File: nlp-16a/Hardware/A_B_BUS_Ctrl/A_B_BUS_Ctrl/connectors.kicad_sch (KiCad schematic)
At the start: 2 parts

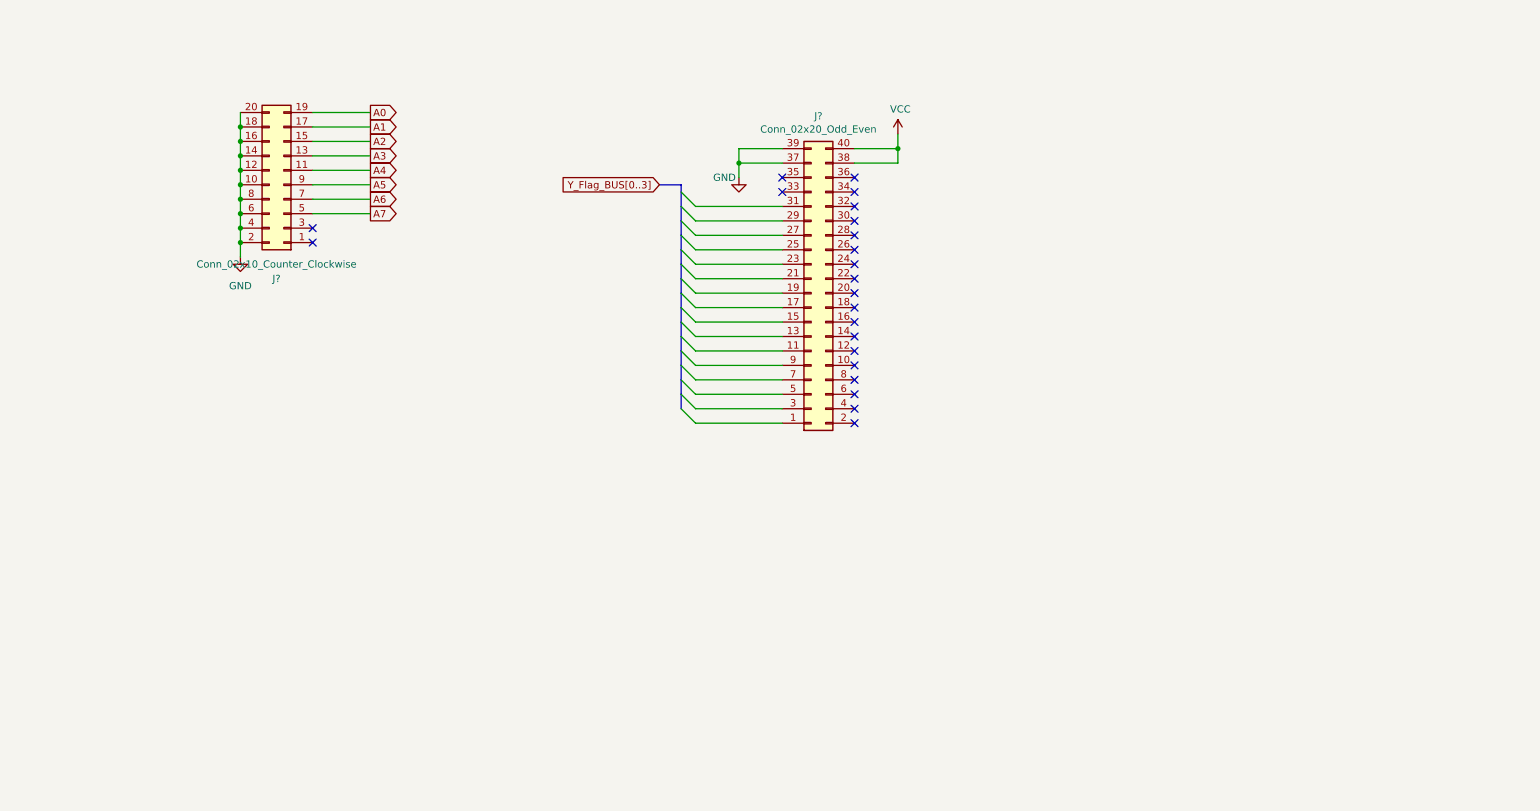
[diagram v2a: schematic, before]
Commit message: 配線作業開始
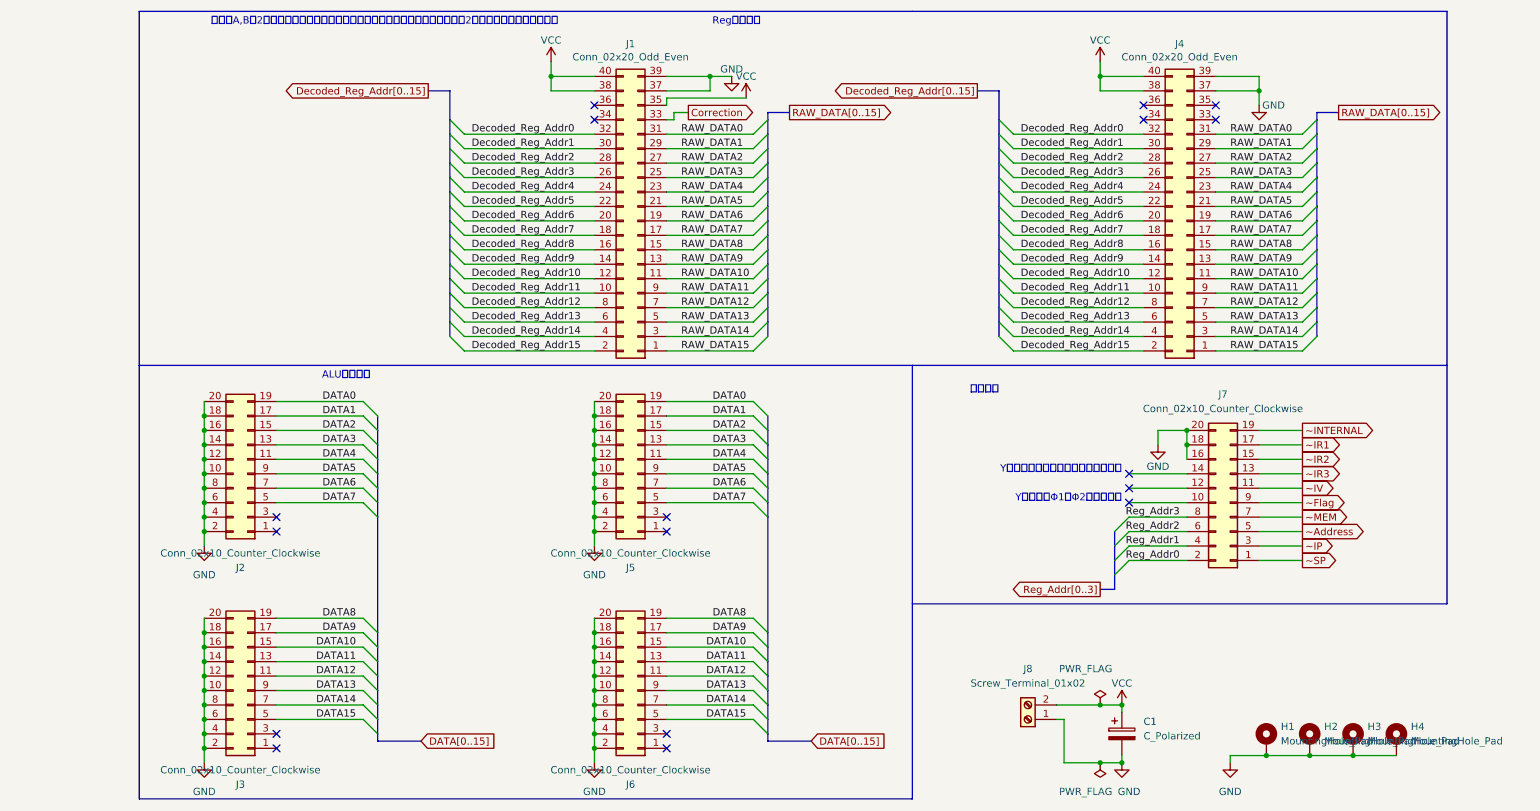
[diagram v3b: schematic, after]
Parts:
- added C1: C_Polarized, Capacitor_THT:CP_Radial_D5.0mm_P2.50mm, symbol Device:C_Polarized
- added H1, H2, H3, H4: MountingHole_Pad, MountingHole:MountingHole_3mm_Pad, symbol Mechanical:MountingHole_Pad
- added J3, J5, J6, J7: Conn_02x10_Counter_Clockwise, Connector_PinHeader_2.54mm:PinHeader_2x10_P2.54mm_Horizontal, symbol Connector_Generic:Conn_02x10_Odd_Even
- added J4: Conn_02x20_Odd_Even, Connector_PinHeader_2.54mm:PinHeader_2x20_P2.54mm_Horizontal, symbol Connector_Generic:Conn_02x20_Odd_Even
- added J8: Screw_Terminal_01x02, TerminalBlock:TerminalBlock_bornier-2_P5.08mm, symbol Connector:Screw_Terminal_01x02
- gave numbers to parts that had none: 2
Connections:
- net GND: now also C1.2, H1.1, H2.1, H3.1, H4.1, J3.10 (Pin_10), J3.12 (Pin_12), J3.14 (Pin_14), J3.16 (Pin_16), J3.18 (Pin_18), J3.2 (Pin_2), J3.20 (Pin_20), J3.4 (Pin_4), J3.6 (Pin_6), J3.8 (Pin_8), J4.37 (Pin_37), J4.39 (Pin_39), J5.10 (Pin_10), J5.12 (Pin_12), J5.14 (Pin_14), J5.16 (Pin_16), J5.18 (Pin_18), J5.2 (Pin_2), J5.20 (Pin_20), J5.4 (Pin_4), J5.6 (Pin_6), J5.8 (Pin_8), J6.10 (Pin_10), J6.12 (Pin_12), J6.14 (Pin_14), J6.16 (Pin_16), J6.18 (Pin_18), J6.2 (Pin_2), J6.20 (Pin_20), J6.4 (Pin_4), J6.6 (Pin_6), J6.8 (Pin_8), J7.16 (Pin_16), J7.18 (Pin_18), J7.20 (Pin_20), J8.1 (Pin_1)
- net VCC: now also J1.35 (Pin_35), C1.1, J4.38 (Pin_38), J4.40 (Pin_40), J8.2 (Pin_2)
- net RAW_DATA15: now reaches J1.1 (Pin_1)
- net RAW_DATA15: now also J4.1 (Pin_1)
- net Decoded_Reg_Addr11: now reaches J1.10 (Pin_10)
- net Decoded_Reg_Addr11: now also J4.10 (Pin_10)
- net RAW_DATA10: now reaches J1.11 (Pin_11)
- net RAW_DATA10: now also J4.11 (Pin_11)
- net Decoded_Reg_Addr10: now reaches J1.12 (Pin_12)
- net Decoded_Reg_Addr10: now also J4.12 (Pin_12)
- net RAW_DATA9: now reaches J1.13 (Pin_13)
- net RAW_DATA9: now also J4.13 (Pin_13)
- net Decoded_Reg_Addr9: now reaches J1.14 (Pin_14)
- net Decoded_Reg_Addr9: now also J4.14 (Pin_14)
- net RAW_DATA8: now reaches J1.15 (Pin_15)
- net RAW_DATA8: now also J4.15 (Pin_15)
- net Decoded_Reg_Addr8: now reaches J1.16 (Pin_16)
- net Decoded_Reg_Addr8: now also J4.16 (Pin_16)
- net RAW_DATA7: now reaches J1.17 (Pin_17)
- net RAW_DATA7: now also J4.17 (Pin_17)
- net Decoded_Reg_Addr7: now reaches J1.18 (Pin_18)
- net Decoded_Reg_Addr7: now also J4.18 (Pin_18)
- net RAW_DATA6: now reaches J1.19 (Pin_19)
- net RAW_DATA6: now also J4.19 (Pin_19)
- net Decoded_Reg_Addr15: now reaches J1.2 (Pin_2)
- net Decoded_Reg_Addr15: now also J4.2 (Pin_2)
- net Decoded_Reg_Addr6: now reaches J1.20 (Pin_20)
- net Decoded_Reg_Addr6: now also J4.20 (Pin_20)
- net RAW_DATA5: now reaches J1.21 (Pin_21)
- net RAW_DATA5: now also J4.21 (Pin_21)
- net Decoded_Reg_Addr5: now reaches J1.22 (Pin_22)
- net Decoded_Reg_Addr5: now also J4.22 (Pin_22)
- net RAW_DATA4: now reaches J1.23 (Pin_23)
- net RAW_DATA4: now also J4.23 (Pin_23)
- net Decoded_Reg_Addr4: now reaches J1.24 (Pin_24)
- net Decoded_Reg_Addr4: now also J4.24 (Pin_24)
- net RAW_DATA3: now reaches J1.25 (Pin_25)
- net RAW_DATA3: now also J4.25 (Pin_25)
- net Decoded_Reg_Addr3: now reaches J1.26 (Pin_26)
- net Decoded_Reg_Addr3: now also J4.26 (Pin_26)
- net RAW_DATA2: now reaches J1.27 (Pin_27)
- net RAW_DATA2: now also J4.27 (Pin_27)
- net Decoded_Reg_Addr2: now reaches J1.28 (Pin_28)
- net Decoded_Reg_Addr2: now also J4.28 (Pin_28)
- net RAW_DATA1: now reaches J1.29 (Pin_29)
- net RAW_DATA1: now also J4.29 (Pin_29)
- net RAW_DATA14: now reaches J1.3 (Pin_3)
- net RAW_DATA14: now also J4.3 (Pin_3)
- net Decoded_Reg_Addr1: now reaches J1.30 (Pin_30)
- net Decoded_Reg_Addr1: now also J4.30 (Pin_30)
- net RAW_DATA0: now reaches J1.31 (Pin_31)
- net RAW_DATA0: now also J4.31 (Pin_31)
- net Decoded_Reg_Addr0: now reaches J1.32 (Pin_32)
- net Decoded_Reg_Addr0: now also J4.32 (Pin_32)
- net Correction: now reaches J1.33 (Pin_33)
- net Decoded_Reg_Addr14: now reaches J1.4 (Pin_4)
- net Decoded_Reg_Addr14: now also J4.4 (Pin_4)
- net RAW_DATA13: now reaches J1.5 (Pin_5)
- net RAW_DATA13: now also J4.5 (Pin_5)
- net Decoded_Reg_Addr13: now reaches J1.6 (Pin_6)
- net Decoded_Reg_Addr13: now also J4.6 (Pin_6)
- net RAW_DATA12: now reaches J1.7 (Pin_7)
- net RAW_DATA12: now also J4.7 (Pin_7)
- net Decoded_Reg_Addr12: now reaches J1.8 (Pin_8)
- net Decoded_Reg_Addr12: now also J4.8 (Pin_8)
- net RAW_DATA11: now reaches J1.9 (Pin_9)
- net RAW_DATA11: now also J4.9 (Pin_9)
- net A0 renamed DATA0
- net DATA0: now also J5.19 (Pin_19)
- net A1 renamed DATA1
- net DATA1: now also J5.17 (Pin_17)
- net A2 renamed DATA2
- net DATA2: now also J5.15 (Pin_15)
- net A3 renamed DATA3
- net DATA3: now also J5.13 (Pin_13)
- net A4 renamed DATA4
- net DATA4: now also J5.11 (Pin_11)
- net A5 renamed DATA5
- net DATA5: now also J5.9 (Pin_9)
- net A6 renamed DATA6
- net DATA6: now also J5.7 (Pin_7)
- net A7 renamed DATA7
- net DATA7: now also J5.5 (Pin_5)
- new net DATA10: J3.15 (Pin_15), J6.15 (Pin_15)
- new net DATA11: J3.13 (Pin_13), J6.13 (Pin_13)
- new net DATA12: J3.11 (Pin_11), J6.11 (Pin_11)
- new net DATA13: J3.9 (Pin_9), J6.9 (Pin_9)
- new net DATA14: J3.7 (Pin_7), J6.7 (Pin_7)
- new net DATA15: J3.5 (Pin_5), J6.5 (Pin_5)
- new net DATA8: J3.19 (Pin_19), J6.19 (Pin_19)
- new net DATA9: J3.17 (Pin_17), J6.17 (Pin_17)
- new net Reg_Addr0: J7.2 (Pin_2)
- new net Reg_Addr1: J7.4 (Pin_4)
- new net Reg_Addr2: J7.6 (Pin_6)
- new net Reg_Addr3: J7.8 (Pin_8)
- new net ~Address: J7.5 (Pin_5)
- new net ~Flag: J7.9 (Pin_9)
- new net ~INTERNAL: J7.19 (Pin_19)
- new net ~IP: J7.3 (Pin_3)
- new net ~IR1: J7.17 (Pin_17)
- new net ~IR2: J7.15 (Pin_15)
- new net ~IR3: J7.13 (Pin_13)
- new net ~IV: J7.11 (Pin_11)
- new net ~MEM: J7.7 (Pin_7)
- new net ~SP: J7.1 (Pin_1)
- no-connect marks 22 -> 17
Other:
- note added: "ALUバス出力"
- note added: "Regバス入力"
- note added: "YバスではΦ1，Φ2で使用する"
- note added: "Yバスでは全レジスタ指定で使用する"
- note added: "バスはA,Bの2パターンあり，それらの基板設計を共通化するためにそれぞれ2つのピンヘッダを設ける．"
- note added: "制御バス"
- moved on the sheet: J1, J2
